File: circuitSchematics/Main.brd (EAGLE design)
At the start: 45.7 x 63.5 mm, 9 parts, among them J1 RASPBERRYPI-40-PIN-GPIO_PTH, J2 Heating_element, Q1 60V/32A/35mΩ, U1 DS18B20

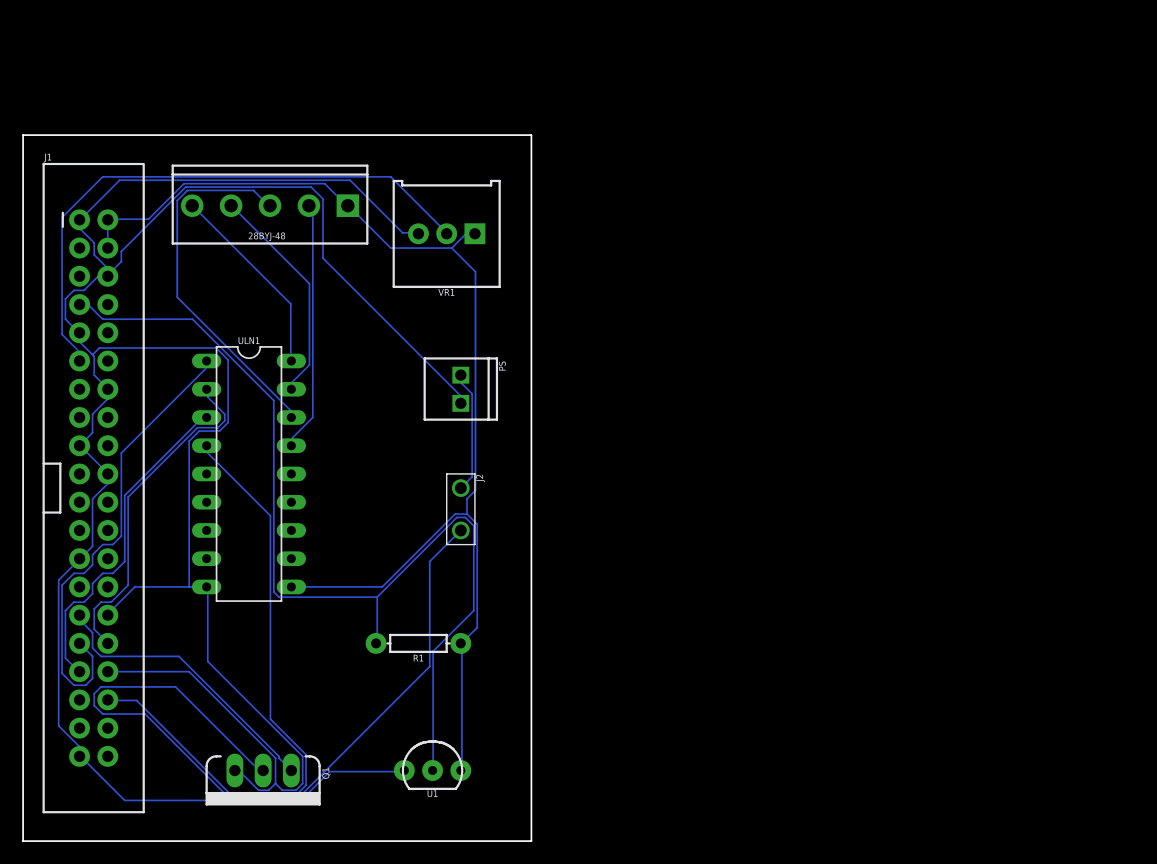
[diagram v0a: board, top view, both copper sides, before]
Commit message: Updated circuit schematics
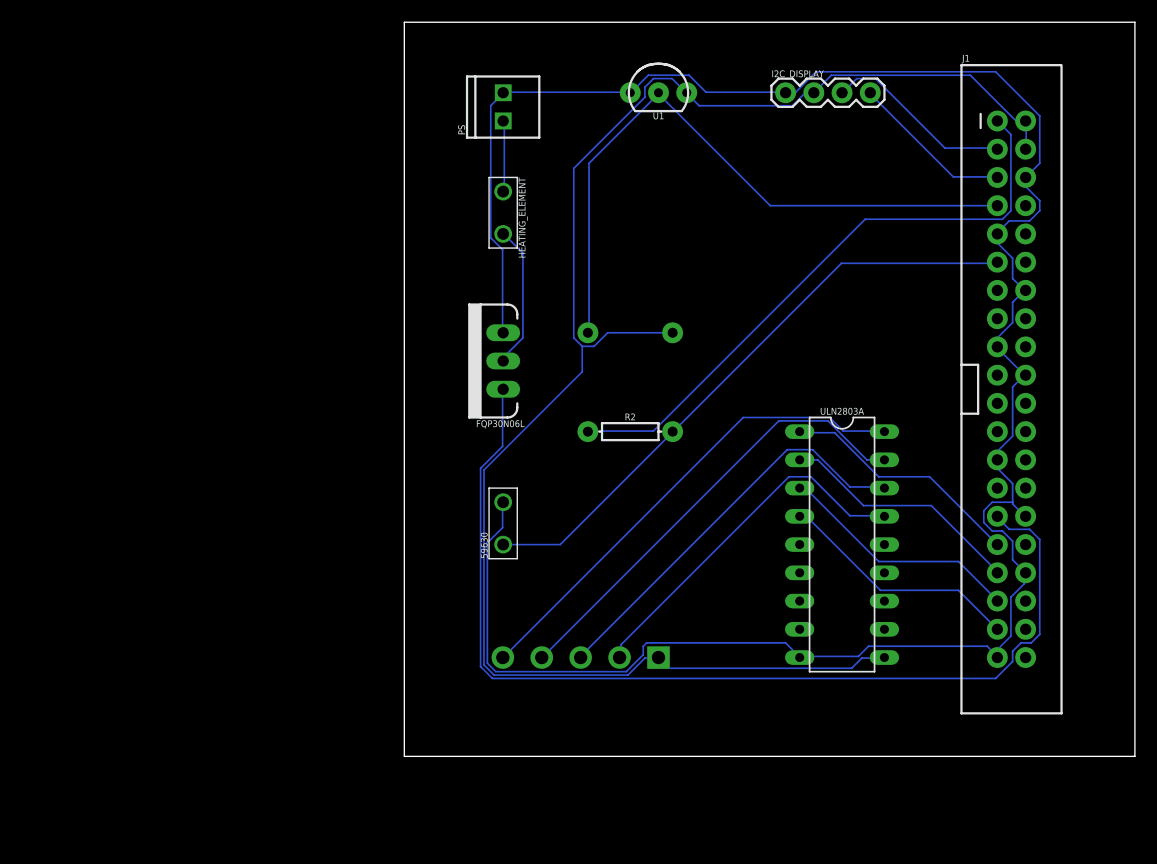
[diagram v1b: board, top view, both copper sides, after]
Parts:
- removed J2: Heating_element, SparkFun-Connectors:1X02_BIG
- removed Q1: 60V/32A/35mΩ, SparkFun-DiscreteSemi:TO220V
- removed ULN1: (no value), SparkFun-IC-Special-Function:DIL18
- removed VR1: 10k, SparkFun-Resistors:TRIMPOT-PTH-3386U
- added 59630, HEATING_ELEMENT: (no value), SparkFun-Connectors:1X02_BIG
- added FQP30N06L: 60V/32A/35mΩ, SparkFun-DiscreteSemi:TO220V
- added I2C_DISPLAY: (no value), SparkFun-Connectors:1X04
- added R2: 10k, SparkFun-Resistors:AXIAL-0.3
- added ULN2803A: (no value), SparkFun-IC-Special-Function:DIL18
- moved J1 83.0 mm to (88.9, 40.6)
- moved U1 64.3 mm to (57.1, 67.3)
- moved 28BYJ-48 49.3 mm to (57.1, 16.5), flipped to the bottom, turned to 0 degrees
- moved R1 33.8 mm to (54.6, 45.7), flipped to the bottom, turned to 0 degrees
- moved PS 23.2 mm to (43.2, 64.8), turned to 90 degrees
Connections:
- net N$1 renamed DQ
- removed net N$12: J1.36, ULN1.4
- removed net N$7: J1.11, VR1.2
- removed net VCC_12V: J2.P$1, PS.P2
- new net 12V: HEATING_ELEMENT.P$1, PS.P2
- new net 3V3: J1.1, R2.P$1
- new net N$5: J1.37, ULN2803A.4
- new net SCL: I2C_DISPLAY.4, J1.5
- new net SDA: I2C_DISPLAY.3, J1.3
- new net WS: 59630.P$1, J1.11, R2.P$2
- net 5V: now also I2C_DISPLAY.2, ULN2803A.10; no longer ULN1.10, VR1.1
- net GND: now also 59630.P$2, FQP30N06L.3, I2C_DISPLAY.1, ULN2803A.9; no longer J1.1, Q1.3, ULN1.9, VR1.3
- net N$10: now also J1.33, ULN2803A.2; no longer J1.32, ULN1.2
- net N$13: now also ULN2803A.18; no longer ULN1.18
- net N$14: now also ULN2803A.17; no longer ULN1.17
- net N$15: now also ULN2803A.16; no longer ULN1.16
- net N$16: now also ULN2803A.15; no longer ULN1.15
- net N$2: now also ULN2803A.1; no longer ULN1.1
- net N$3: now also FQP30N06L.1; no longer Q1.1
- net N$4: now also J1.35, ULN2803A.3; no longer J1.33, ULN1.3
- net N$8: now also FQP30N06L.2, HEATING_ELEMENT.P$2; no longer J2.P$2, Q1.2
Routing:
- net N$3: track 26.0 -> 92.0 mm
- net GND: track 267.2 -> 203.4 mm
- net N$8: track 71.5 -> 12.9 mm
- net N$12: track 55.9 -> 0.00 mm
- net WS: track 0.00 -> 55.0 mm
- net 3V3: track 0.00 -> 54.8 mm
- net N$7: track 51.8 -> 0.00 mm
- net 5V: track 107.7 -> 146.1 mm
- net DQ: track 87.5 -> 58.9 mm
- net N$13: track 17.7 -> 43.8 mm
- net N$5: track 0.00 -> 22.0 mm
- net N$14: track 20.1 -> 41.1 mm
- net N$2: track 41.6 -> 22.0 mm
- net SDA: track 0.00 -> 17.2 mm
- net SCL: track 0.00 -> 14.7 mm
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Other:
- board size 45.7 x 63.5 mm -> 65.7 x 66 mm
